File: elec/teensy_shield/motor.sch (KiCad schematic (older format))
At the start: 0 parts

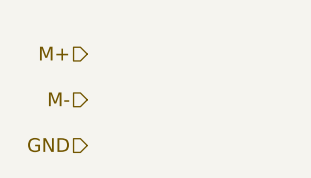
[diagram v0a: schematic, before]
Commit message: Completed new board schematics.
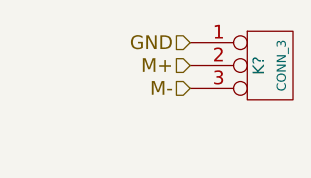
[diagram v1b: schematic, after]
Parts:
- added K?: CONN_3, symbol CONN_3
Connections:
- net GND: now also K?.1 (P1)
- net M+: now also K?.2 (PM)
- net M-: now also K?.3 (P3)
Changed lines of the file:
@@
 LIBS:contrib
 LIBS:valves
+LIBS:arduino_shieldsNCL
+LIBS:teensy
+LIBS:pololu
+LIBS:teensy_shield-cache
 EELAYER 24 0
 EELAYER END
 $Descr A4 11693 8268
 encoding utf-8
-Sheet 6 26
+Sheet 7 34
 Title ""
 Date ""
@@
 Comment4 ""
 $EndDescr
-Text HLabel 4750 3200 0    60   Input ~ 0
+Text HLabel 5200 3250 0    60   Input ~ 0
 M+
-Text HLabel 4750 3400 0    60   Input ~ 0
+Text HLabel 5200 3350 0    60   Input ~ 0
 M-
-Text HLabel 4750 3600 0    60   Input ~ 0
+Text HLabel 5200 3150 0    60   Input ~ 0
 GND
+$Comp
+L CONN_3 K?
+U 1 1 55E8223E
+P 5550 3250
+F 0 "K?" V 5500 3250 50  0000 C CNN
+F 1 "CONN_3" V 5600 3250 40  0000 C CNN
+F 2 "" H 5550 3250 60  0000 C CNN
+F 3 "" H 5550 3250 60  0000 C CNN
+	1    5550 3250
+	1    0    0    -1
+$EndComp
 $EndSCHEMATC

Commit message: Elec ?
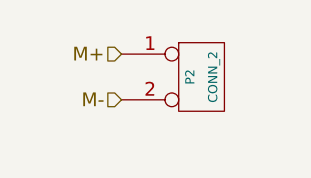
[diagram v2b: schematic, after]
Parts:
- removed K?: CONN_3, symbol CONN_3
- added P7: CONN_2, symbol CONN_2
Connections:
- net M+: now also P7.1 (P1)
- net M-: now also P7.2 (PM)
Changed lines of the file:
@@
 Comment4 ""
 $EndDescr
-Text HLabel 5200 3250 0    60   Input ~ 0
+Text HLabel 4900 3200 0    60   Input ~ 0
 M+
-Text HLabel 5200 3350 0    60   Input ~ 0
+Text HLabel 4900 3400 0    60   Input ~ 0
 M-
-Text HLabel 5200 3150 0    60   Input ~ 0
-GND
 $Comp
-L CONN_3 K?
-U 1 1 55E8223E
-P 5550 3250
-F 0 "K?" V 5500 3250 50  0000 C CNN
-F 1 "CONN_3" V 5600 3250 40  0000 C CNN
-F 2 "" H 5550 3250 60  0000 C CNN
-F 3 "" H 5550 3250 60  0000 C CNN
-	1    5550 3250
+L CONN_2 P7
+U 1 1 55E7454A
+P 5250 3300
+AR Path="/55E6307C/55E6315B/55E7454A" Ref="P7"  Part="1"
+AR Path="/55E7381B/55E6315B/55E7454A" Ref="P2"  Part="1"
+AR Path="/55E7381C/55E6315B/55E7454A" Ref="P3"  Part="1"
+AR Path="/55E7381D/55E6315B/55E7454A" Ref="P4"  Part="1"
+F 0 "P2" V 5200 3300 40  0000 C CNN
+F 1 "CONN_2" V 5300 3300 40  0000 C CNN
+F 2 "" H 5250 3300 60  0000 C CNN
+F 3 "" H 5250 3300 60  0000 C CNN
+	1    5250 3300
 	1    0    0    -1
 $EndComp
